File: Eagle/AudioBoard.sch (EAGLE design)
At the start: 7 parts, among them M1 WIRELESS-NRF24L01, U1 NC7SZ157P6X

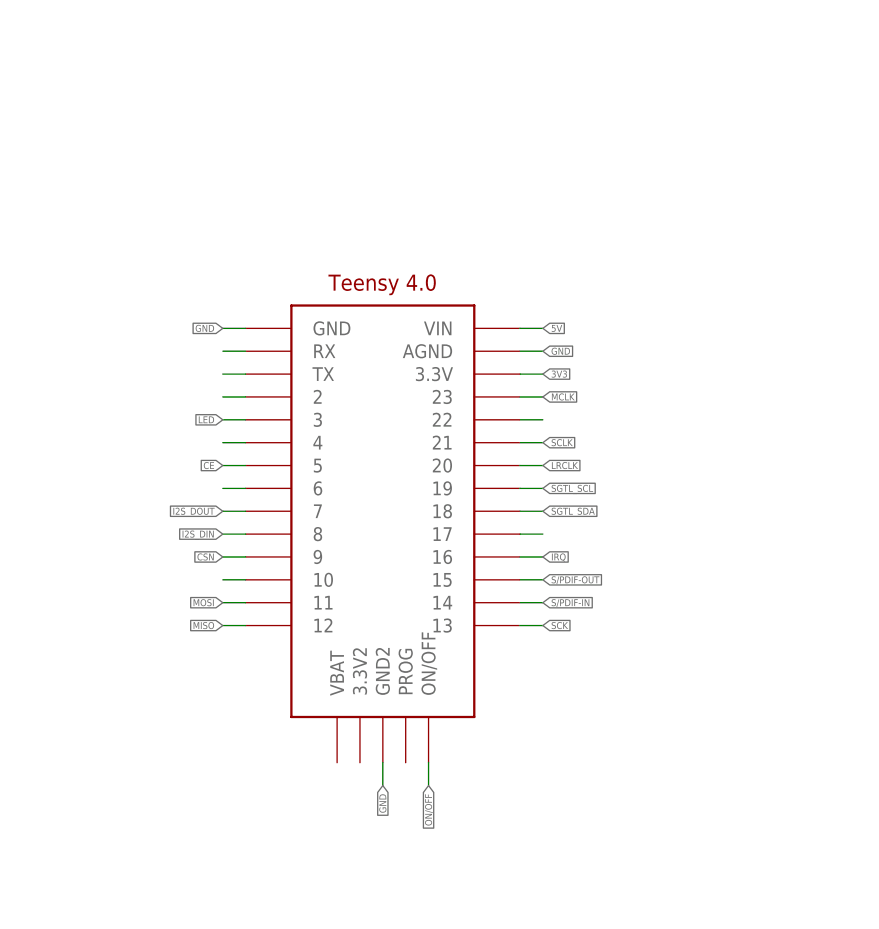
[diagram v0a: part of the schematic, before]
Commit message: schematic and board file work.
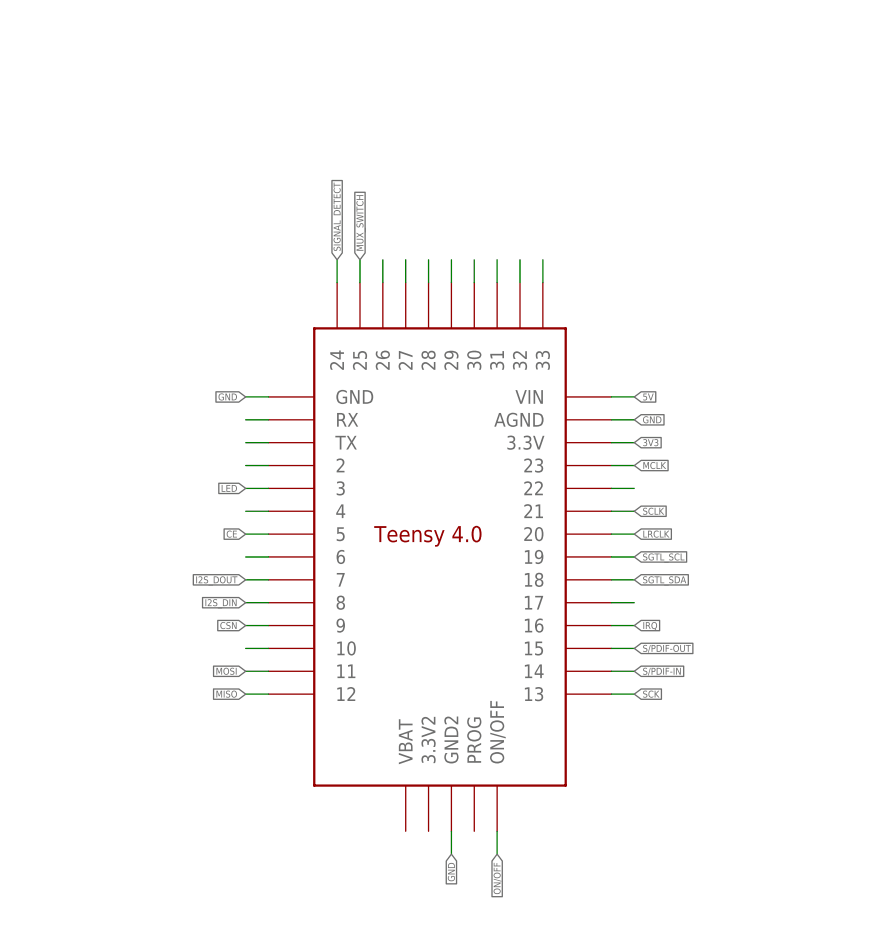
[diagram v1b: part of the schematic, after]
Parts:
- removed U$1: TEENSY4.0, Teensy3.2:TEENSY4.0
- added U$5: TEENSY4.0_FULL_IO, Teensy3.2:TEENSY4.0_FULL_IO
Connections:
- removed net N$1: U$1.RX
- removed net N$11: U$1.10
- removed net N$18: U$1.17
- removed net N$2: U$1.TX
- removed net N$23: U$1.22
- removed net N$3: U$1.2
- removed net N$5: U$1.4
- removed net N$7: U$1.6
- new net N$10: U$5.22
- new net N$16: U$5.17
- new net N$28: U$5.10
- new net N$32: U$5.6
- new net N$34: U$5.4
- new net N$36: U$5.2
- new net N$37: U$5.TX
- new net N$38: U$5.RX
- new net N$42: U$5.26
- new net N$43: U$5.27
- new net N$44: U$5.28
- new net N$45: U$5.29
- new net N$46: U$5.30
- new net N$47: U$5.31
- new net N$48: U$5.32
- new net N$49: U$5.33
- net 3V3: now also U$5.3.3V; no longer U$1.3.3V
- net 5V: now also U$5.VIN; no longer U$1.VIN
- net CE: now also U$5.5; no longer U$1.5
- net CSN: now also U$5.9; no longer U$1.9
- net GND: now also U$5.AGND, U$5.GND, U$5.GND2; no longer U$1.AGND, U$1.GND, U$1.GND2
- net I2S_DIN: now also U$5.8; no longer U$1.8
- net I2S_DOUT: now also U$5.7; no longer U$1.7
- net IRQ: now also U$5.16; no longer U$1.16
- net LED: now also U$5.3; no longer U$1.3
- net LRCLK: now also U$5.20; no longer U$1.20
- net MCLK: now also U$5.23; no longer U$1.23
- net MISO: now also U$5.12; no longer U$1.12
- net MOSI: now also U$5.11; no longer U$1.11
- net MUX_SWITCH: now also U$5.25
- net ON/OFF: now also U$5.ON/OFF; no longer U$1.ON/OFF
- net S/PDIF-IN: now also U$5.14; no longer U$1.14
- net S/PDIF-OUT: now also U$5.15; no longer U$1.15
- net SCK: now also U$5.13; no longer U$1.13
- net SCLK: now also U$5.21; no longer U$1.21
- net SGTL_SCL: now also U$5.19; no longer U$1.19
- net SGTL_SDA: now also U$5.18; no longer U$1.18
- net SIGNAL_DETECT: now also U$5.24

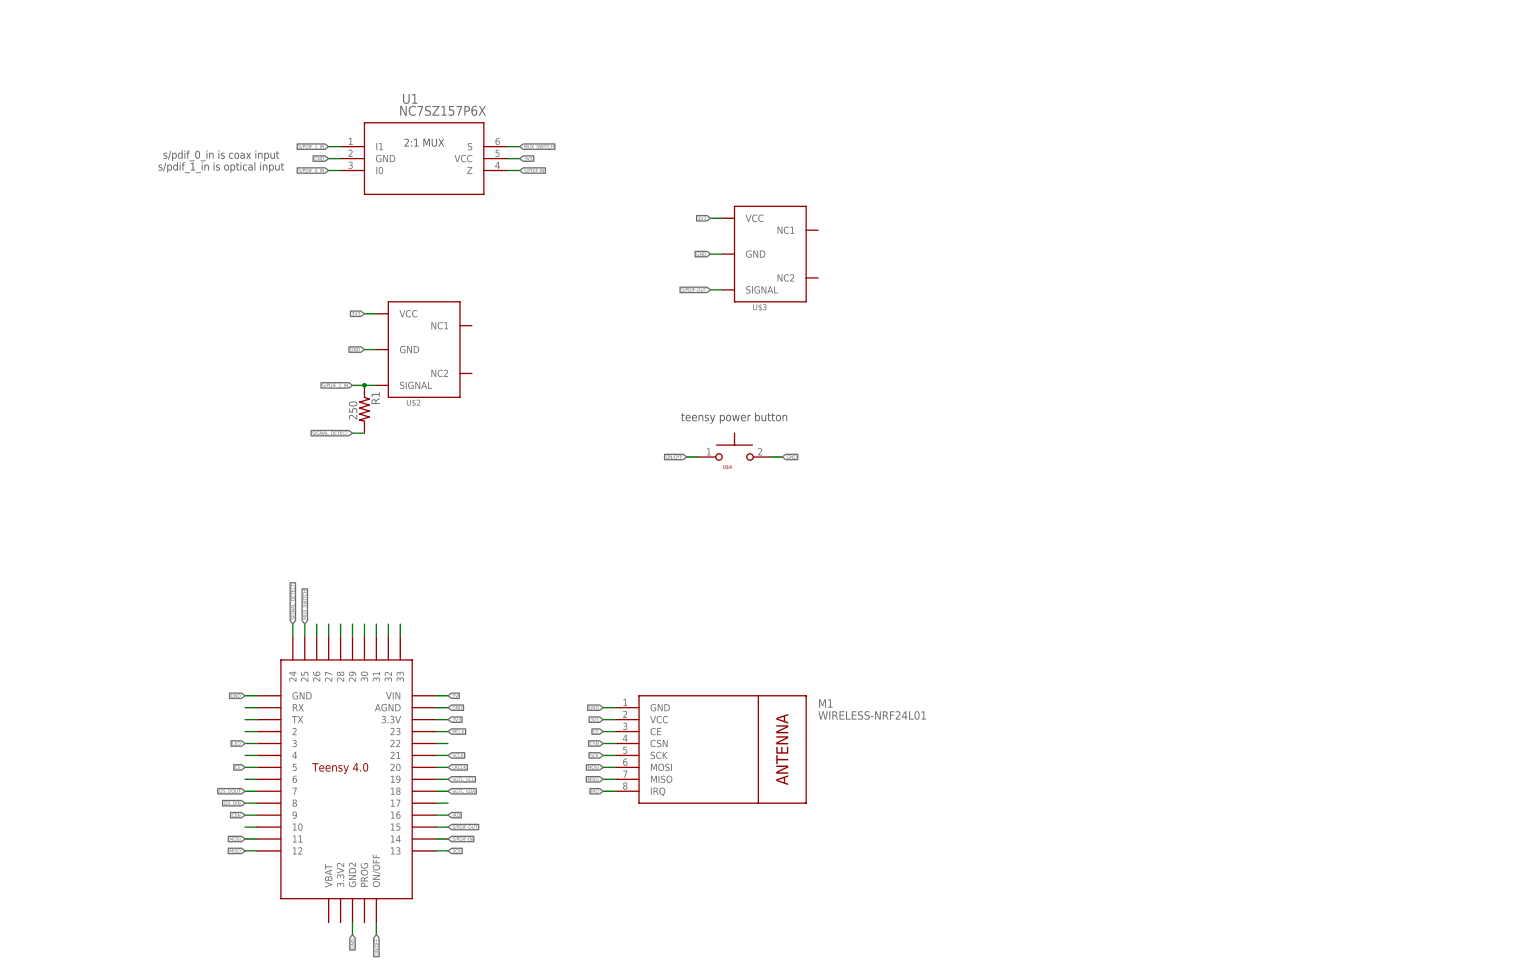
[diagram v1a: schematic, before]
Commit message: updates to eagle files
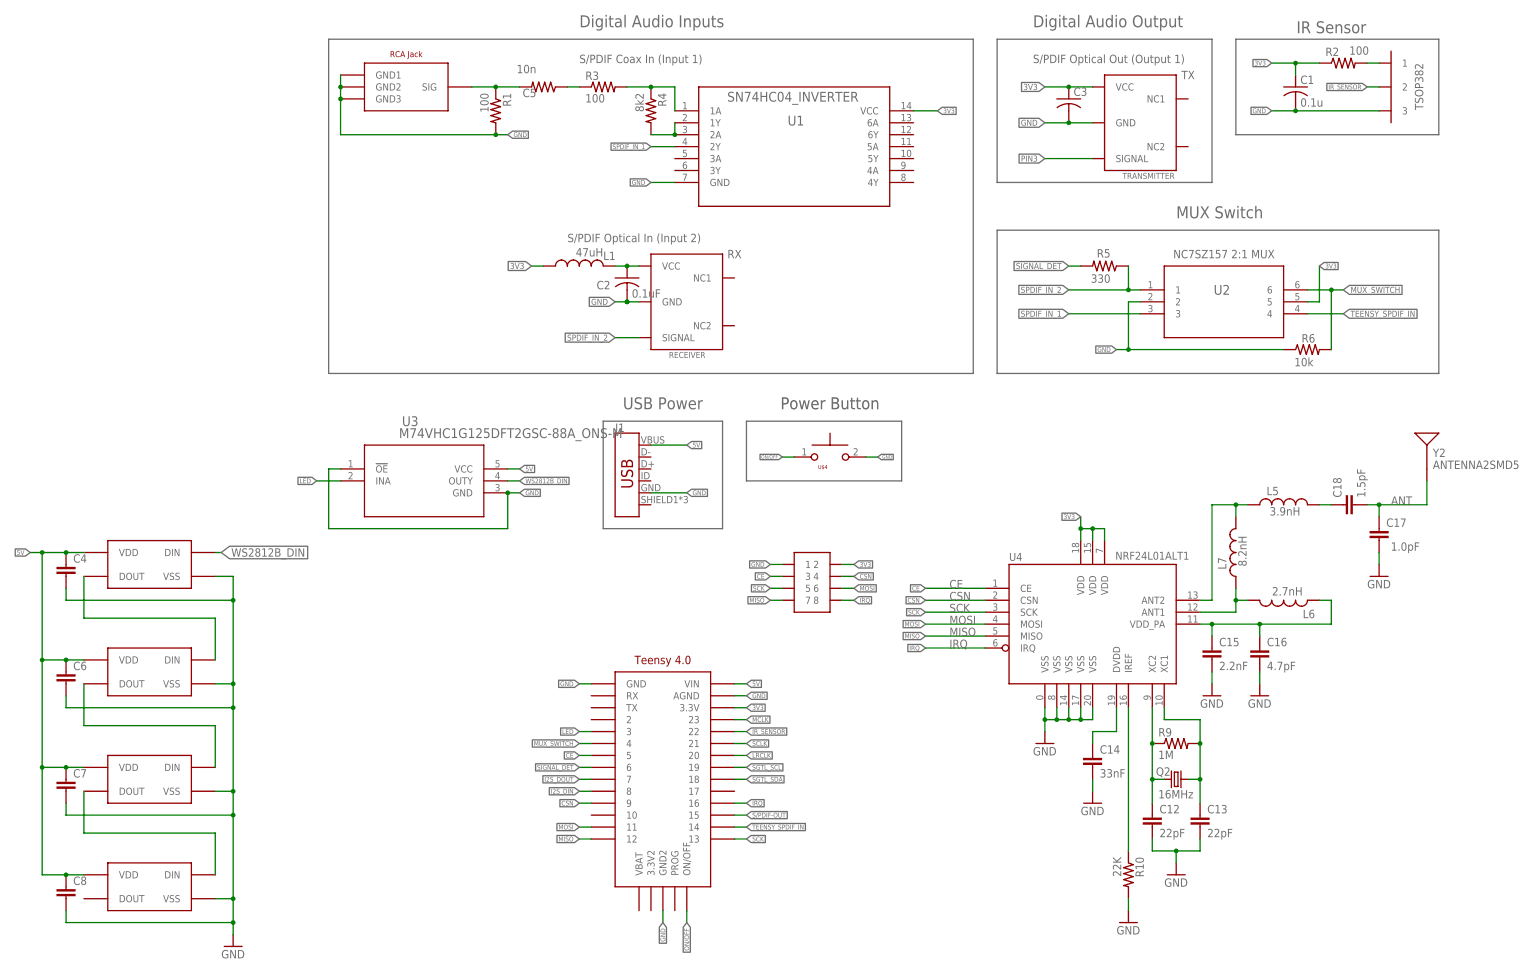
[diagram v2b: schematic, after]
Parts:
- removed M1: WIRELESS-NRF24L01, NRF24L01:WIRELESS-NRF24L01
- added C1: 0.1u, rcl:C-USC0603K
- added C12, C13: 22pF, SparkFun:CAP0402-CAP
- added C14: 33nF, SparkFun:CAP0402-CAP
- added C15: 2.2nF, SparkFun:CAP0402-CAP
- added C16: 4.7pF, SparkFun:CAP0402-CAP
- added C17: 1.0pF, SparkFun:CAP0402-CAP
- added C18: 1.5pF, SparkFun:CAP0402-CAP
- added C2: 0.1uF, rcl:C-USC0603
- added C3: (no value), rcl:C-USC0603
- added C4, C6, C7, C8: (no value), resistor:C-EUC0603
- added C5: 10n, resistor:R-US_R0603
- added J1: (no value), SparkFun-Connectors:USB_MICRO-BREDUCED_PASTE
- added L1: 47uH, resistor:L-USL2012C
- added L5: 3.9nH, SparkFun:INDUCTOR0402
- added L6: 2.7nH, SparkFun:INDUCTOR0402
- added L7: 8.2nH, SparkFun:INDUCTOR0402
- added Q2: 16MHz, SparkFun:CRYSTAL5X3
- added R10: 22K, SparkFun:RESISTOR0402-RES
- added R2, R3: 100, resistor:R-US_R0603
- added R4: 8k2, resistor:R-US_R0603
- added R5: 330, rcl:R-US_R0603
- added R6: 10k, rcl:R-US_R0603
- added R9: 1M, SparkFun:RESISTOR0402-RES
- added RECEIVER: S/PDIF-IN, SPDIF:S/PDIF-IN
- added TRANSMITTER: S/PDIF-OUT, SPDIF:S/PDIF-OUT
- added U$1: 1X3HEADER, 1x2HEADER:1X3HEADER
- added U$6, U$7, U$8: WS2812B, Neopixel WS2812B:WS2812B
- added U$9: 2X4HEADER, 1x2HEADER:2X4HEADER
- added U2: 2:1_MUX_NC7SZ157P6X, AudioSwitch:2:1_MUX_NC7SZ157P6X
- added U3: M74VHC1G125DFT2GSC-88A_ONS-M, AudioSwitch:M74VHC1G125DFT2GSC-88A_ONS-M
- added U4: NRF24L01ALT1, Testing:NRF24L01ALT1
- added Y2: ANTENNA2SMD5, SparkFun:ANTENNA2SMD5
- R1: value 250 -> 100; device resistor:R-US_R0805 -> resistor:R-US_R0603
- U$2: value S/PDIF-IN -> RCA_JACK; device SPDIF:S/PDIF-IN -> COAX_SPDIF:RCA_JACK
- U$3: value S/PDIF-OUT -> TEENSY4.0; device SPDIF:S/PDIF-OUT -> Teensy3.2:TEENSY4.0
- U$5: value TEENSY4.0_FULL_IO -> WS2812B; device Teensy3.2:TEENSY4.0_FULL_IO -> Neopixel WS2812B:WS2812B
- U1: value NC7SZ157P6X -> SN74HC04_INVERTER; device MUX_2-1_NC7SZ157P6X:NC7SZ157P6X -> COAX_SPDIF:SN74HC04_INVERTER
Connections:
- removed net N$10: U$5.22
- removed net N$28: U$5.10
- removed net N$32: U$5.6
- removed net N$34: U$5.4
- removed net N$36: U$5.2
- removed net N$37: U$5.TX
- removed net N$38: U$5.RX
- removed net N$42: U$5.26
- removed net N$43: U$5.27
- removed net N$44: U$5.28
- removed net N$45: U$5.29
- removed net N$46: U$5.30
- removed net N$47: U$5.31
- removed net N$48: U$5.32
- removed net N$49: U$5.33
- removed net S/PDIF-IN: U$5.14, U1.Z
- removed net S/PDIF_0_IN: U1.I0
- removed net S/PDIF_1_IN: R1.1, U$2.SIGNAL, U1.I1
- removed net SIGNAL_DETECT: R1.2, U$5.24
- new net 1TO2: U$5.DOUT, U$6.DIN
- new net 2TO3: U$6.DOUT, U$7.DIN
- new net 3TO4: U$7.DOUT, U$8.DIN
- new net ANT: C17.2, C18.2, Y2.SIGNAL
- new net IR_SENSOR: U$1.2, U$3.22
- new net N$1: C5.2, R1.1, U$2.SIG
- new net N$15: C12.1, Q2.1, R9.1, U4.XC2
- new net N$17: L5.1, L7.2, U4.ANT2
- new net N$18: C15.1, C16.1, L6.1, U4.VDD_PA
- new net N$19: R10.1, U4.IREF
- new net N$2: R2.2, U$1.1
- new net N$20: C14.1, U4.DVDD
- new net N$21: L6.2, L7.1, U4.ANT1
- new net N$22: C18.1, L5.2
- new net N$3: C5.1, R3.1
- new net N$4: R3.2, R4.1, U1.1A
- new net N$5: C2.1, L1.2, RECEIVER.VCC
- new net N$6: R4.2, U1.1Y, U1.2A
- new net PIN3: TRANSMITTER.SIGNAL
- new net SIGNAL_DET: R5.2, U$3.6
- new net SPDIF_IN_1: U1.2Y, U2.3
- new net SPDIF_IN_2: R5.1, RECEIVER.SIGNAL, U2.1
- new net TEENSY_SPDIF_IN: U$3.14, U2.4
- new net WS2812B_DIN: U$5.DIN, U3.OUTY
- net 3V3: now also C1.1, C3.1, L1.1, R2.1, TRANSMITTER.VCC, U$3.3.3V, U$9.2, U2.5, U4.VDD@15, U4.VDD@18, U4.VDD@7; no longer M1.VCC, U$2.VCC, U$3.VCC, U$5.3.3V
- net 5V: now also C4.1, C6.1, C7.1, C8.1, J1.VBUS, U$3.VIN, U$5.VDD, U$6.VDD, U$7.VDD, U$8.VDD, U3.VCC; no longer U$5.VIN
- net CE: now also U$3.5, U$9.3, U4.CE; no longer M1.CE, U$5.5
- net CSN: now also U$3.9, U$9.4, U4.CSN; no longer M1.CSN, U$5.9
- net GND: now also C1.2, C12.2, C13.2, C14.2, C15.2, C16.2, C17.1, C2.2, C3.2, C4.2, C6.2, C7.2, C8.2, J1.GND, R1.2, R10.2, R6.1, RECEIVER.GND, TRANSMITTER.GND, U$1.3, U$2.GND1, U$2.GND2, U$2.GND3, U$3.AGND, U$3.GND2, U$5.VSS, U$6.VSS, U$7.VSS, U$8.VSS, U$9.1, U2.2, U3.!OE, U3.GND, U4.VSS@0, U4.VSS@14, U4.VSS@17, U4.VSS@20, U4.VSS@8; no longer M1.GND, U$2.GND, U$5.AGND, U$5.GND, U$5.GND2
- net I2S_DIN: now also U$3.8; no longer U$5.8
- net I2S_DOUT: now also U$3.7; no longer U$5.7
- net IRQ: now also U$3.16, U$9.8, U4.IRQ; no longer M1.IRQ, U$5.16
- net LED: now also U$3.3, U3.INA; no longer U$5.3
- net LRCLK: now also U$3.20; no longer U$5.20
- net MCLK: now also U$3.23; no longer U$5.23
- net MISO: now also U$3.12, U$9.7, U4.MISO; no longer M1.MISO, U$5.12
- net MOSI: now also U$3.11, U$9.6, U4.MOSI; no longer M1.MOSI, U$5.11
- net MUX_SWITCH: now also R6.2, U$3.4, U2.6; no longer U$5.25, U1.S
- net N$16: now also C13.1, Q2.2, R9.2, U4.XC1; no longer U$5.17
- net ON/OFF: now also U$3.ON/OFF; no longer U$5.ON/OFF
- net S/PDIF-OUT: now also U$3.15; no longer U$3.SIGNAL, U$5.15
- net SCK: now also U$3.13, U$9.5, U4.SCK; no longer M1.SCK, U$5.13
- net SCLK: now also U$3.21; no longer U$5.21
- net SGTL_SCL: now also U$3.19; no longer U$5.19
- net SGTL_SDA: now also U$3.18; no longer U$5.18
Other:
- note added: "Digital Audio Inputs"
- note added: "Digital Audio Output"
- note added: "IR Sensor"
- note added: "MUX Switch"
- note added: "NC7SZ157 2:1 MUX"
- note added: "Power Button"
- note added: "RX"
- note added: "S/PDIF Coax In (Input 1)"
- note added: "S/PDIF Optical In (Input 2)"
- note added: "S/PDIF Optical Out (Output 1)"
- note added: "TSOP382"
- note added: "TX"
- note added: "USB Power"
- note removed: "2:1 MUX"
- note removed: "s/pdif_0_in is coax input s/pdif_1_in is optical input"
- note removed: "teensy power button"
- moved on the sheet: R1, U$4
